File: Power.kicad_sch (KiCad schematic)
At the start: 22 parts, among them IC1 LM74502HDDFR, Q2 NVMFWS1D7N04XMT1G, U4 LMR33630ADDA

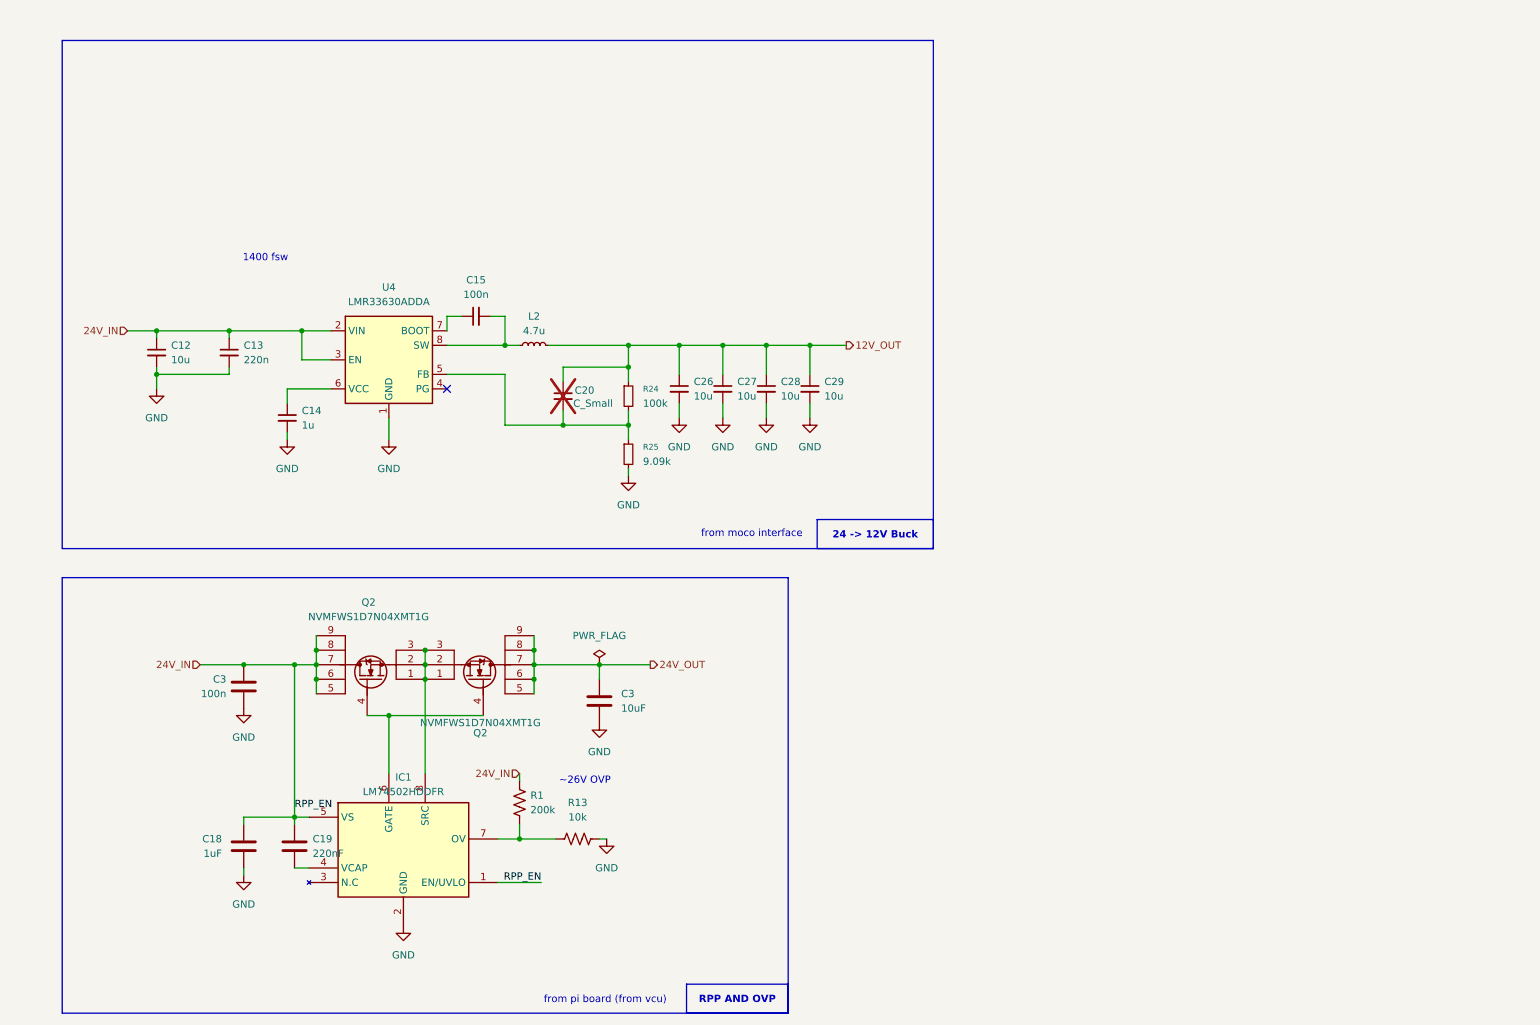
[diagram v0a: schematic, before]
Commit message: schem review changes
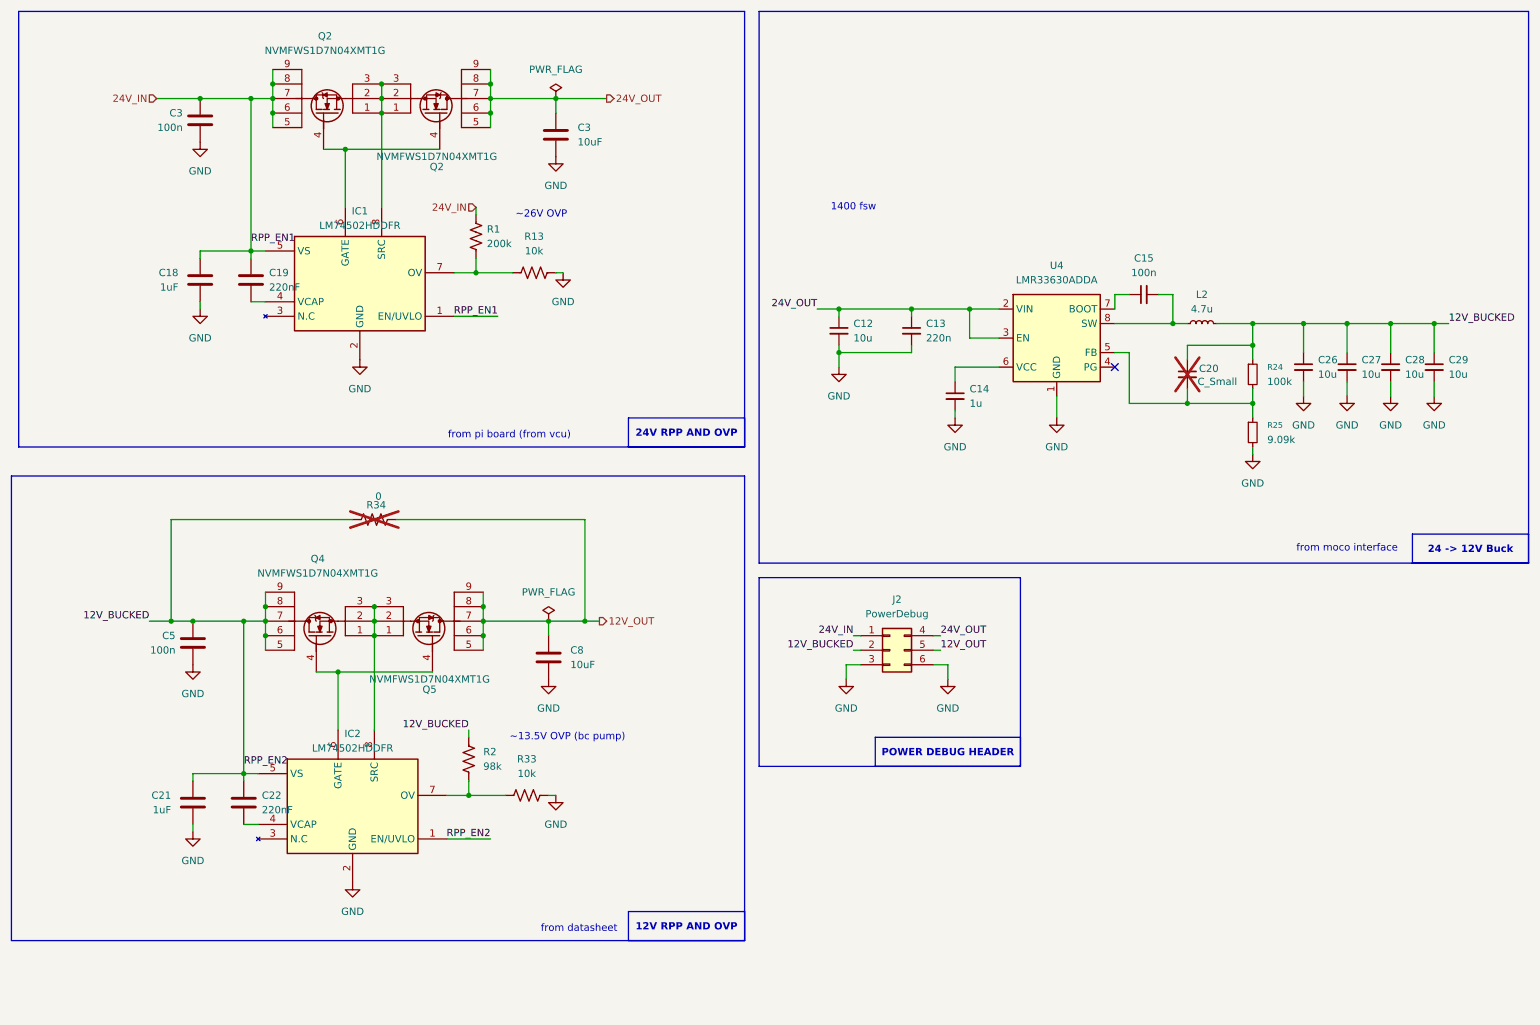
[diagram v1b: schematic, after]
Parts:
- added C21: 1uF, Capacitor_SMD:C_0805_2012Metric_Pad1.18x1.45mm_HandSolder, symbol Device:C
- added C22: 220nF, Capacitor_SMD:C_0805_2012Metric_Pad1.18x1.45mm_HandSolder, symbol Device:C
- added C5: 100n, Capacitor_SMD:C_0603_1608Metric_Pad1.08x0.95mm_HandSolder, symbol Device:C
- added C8: 10uF, Capacitor_SMD:C_0805_2012Metric_Pad1.18x1.45mm_HandSolder, symbol Device:C
- added IC2: LM74502HDDFR, UTSVT_Power_SP:SOT65P280X110-8N, symbol UTSVT_ICs:LM74502HDDFR
- added J2: PowerDebug, Connector_PinHeader_2.54mm:PinHeader_2x03_P2.54mm_Vertical, symbol Connector_Generic:Conn_02x03_Top_Bottom
- added Q4, Q5: NVMFWS1D7N04XMT1G, Controls_Pi:NVMFWS3D0P04M8LT1G, symbol NVMFWS1D7N04XMT1G:NVMFWS1D7N04XMT1G
- added R2: 98k, Resistor_SMD:R_0603_1608Metric_Pad0.98x0.95mm_HandSolder, symbol Device:R_US
- added R33: 10k, Resistor_SMD:R_0603_1608Metric_Pad0.98x0.95mm_HandSolder, symbol Device:R_US
- added R34: 0, Resistor_SMD:R_0603_1608Metric, symbol Device:R_US
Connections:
- net 12V_OUT: now also C8.1, J2.5 (Pin_5), Q5.5, Q5.6, Q5.7, Q5.8, Q5.9, R34.2; no longer C20.1, C26.1, C27.1, C28.1, C29.1, L2.2, R24.1
- net 24V_IN: now also J2.1 (Pin_1); no longer C12.1, C13.1, U4.2 (VIN), U4.3 (EN)
- net 24V_OUT: now also C12.1, C13.1, U4.2 (VIN), U4.3 (EN), J2.4 (Pin_4)
- net GND: now also C21.1, C5.1, C8.2, IC2.2 (GND), J2.3 (Pin_3), J2.6 (Pin_6), R33.2
- new net: IC2.8 (SRC), Q4.1, Q4.2, Q4.3, Q5.1, Q5.2, Q5.3
- new net: IC2.6 (GATE), Q4.4, Q5.4
- new net: C22.2, IC2.4 (VCAP)
- new net: IC2.7 (OV), R2.2, R33.1
- new net 12V_BUCKED: C20.1, C21.2, C22.1, C26.1, C27.1, C28.1, C29.1, C5.2, IC2.1 (EN/UVLO), IC2.5 (VS), J2.2 (Pin_2), L2.2, Q4.5, Q4.6, Q4.7, Q4.8, Q4.9, R2.1, R24.1, R34.1
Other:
- note added: "from datasheet"
- note added: "~13.5V OVP (bc pump)"
- moved on the sheet: C12, C13, C14, C15, C18, C19, C20, C26, C27, C28, C29, C3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
